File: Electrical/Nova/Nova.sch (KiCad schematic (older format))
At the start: 0 parts

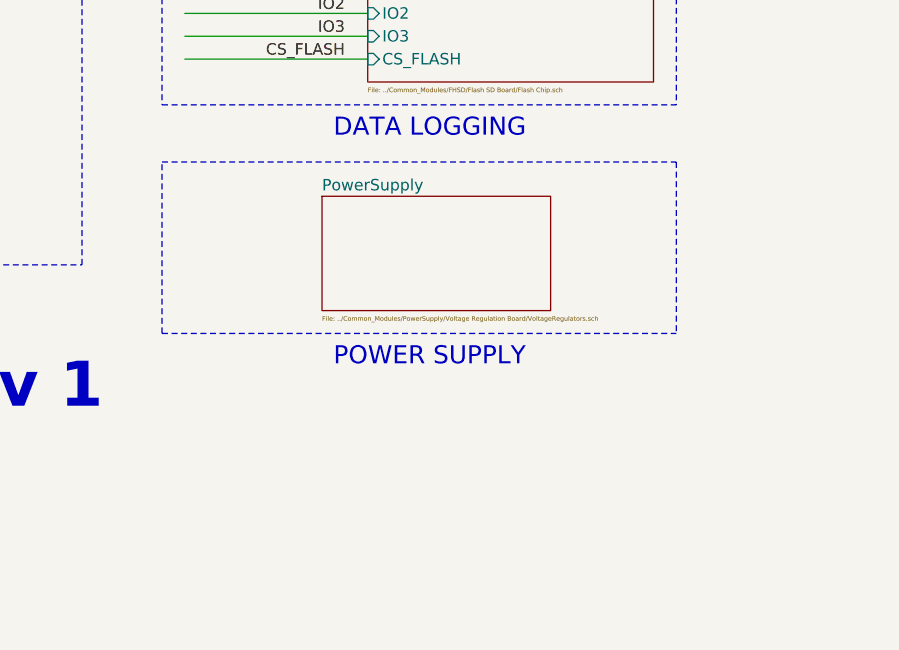
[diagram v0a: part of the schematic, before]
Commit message: Crossing Fingers Github
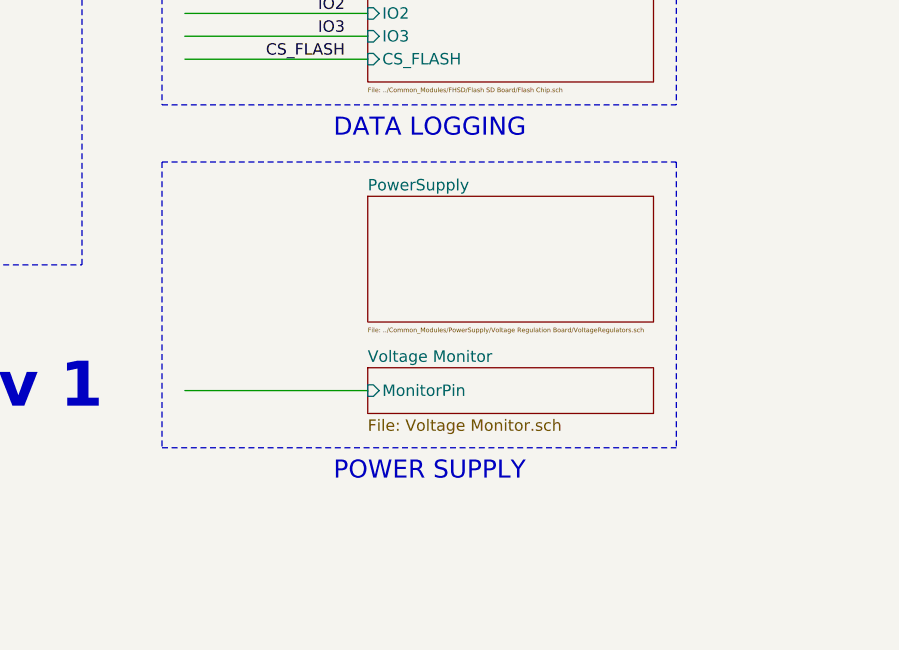
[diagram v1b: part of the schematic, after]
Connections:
- wire segments 101 -> 102
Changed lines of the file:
@@
 $Descr USLetter 11000 8500
 encoding utf-8
-Sheet 1 21
+Sheet 1 22
 Title ""
 Date ""
@@
 	8000 3050 10250 3050
 Wire Notes Line
-	10250 4900 10250 5650
-Wire Notes Line
 	750  6200 3000 6200
 Wire Notes Line
@@
 Wire Wire Line
 	2150 2450 2900 2450
-Wire Notes Line
-	8000 5650 8000 4900
-Text Notes 8750 5800 0    79   ~ 0
+Text Notes 8750 6300 0    79   ~ 0
 POWER SUPPLY\n
 $Sheet
-S 8700 5050 1000 500
+S 8900 5050 1250 550
 U 5F3B0B4B
 F0 "PowerSupply" 50
@@
 	8000 4900 10250 4900
 Wire Notes Line
-	8000 5650 10250 5650
+	8000 6150 10250 6150
 NoConn ~ 10150 1600
 NoConn ~ 10150 1700
@@
 Text Label 8800 1050 2    50   ~ 0
 MOSI
+$Sheet
+S 8900 5800 1250 200
+U 5F964042
+F0 "Voltage Monitor" 50
+F1 "Voltage Monitor.sch" 50
+F2 "MonitorPin" I L 8900 5900 50
+$EndSheet
+Wire Notes Line
+	10250 4900 10250 6150
+Wire Notes Line
+	8000 4900 8000 6150
+Wire Wire Line
+	8900 5900 8100 5900
 $EndSCHEMATC
